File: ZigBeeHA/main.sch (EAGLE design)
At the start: 12 parts, among them IC1 REG1117

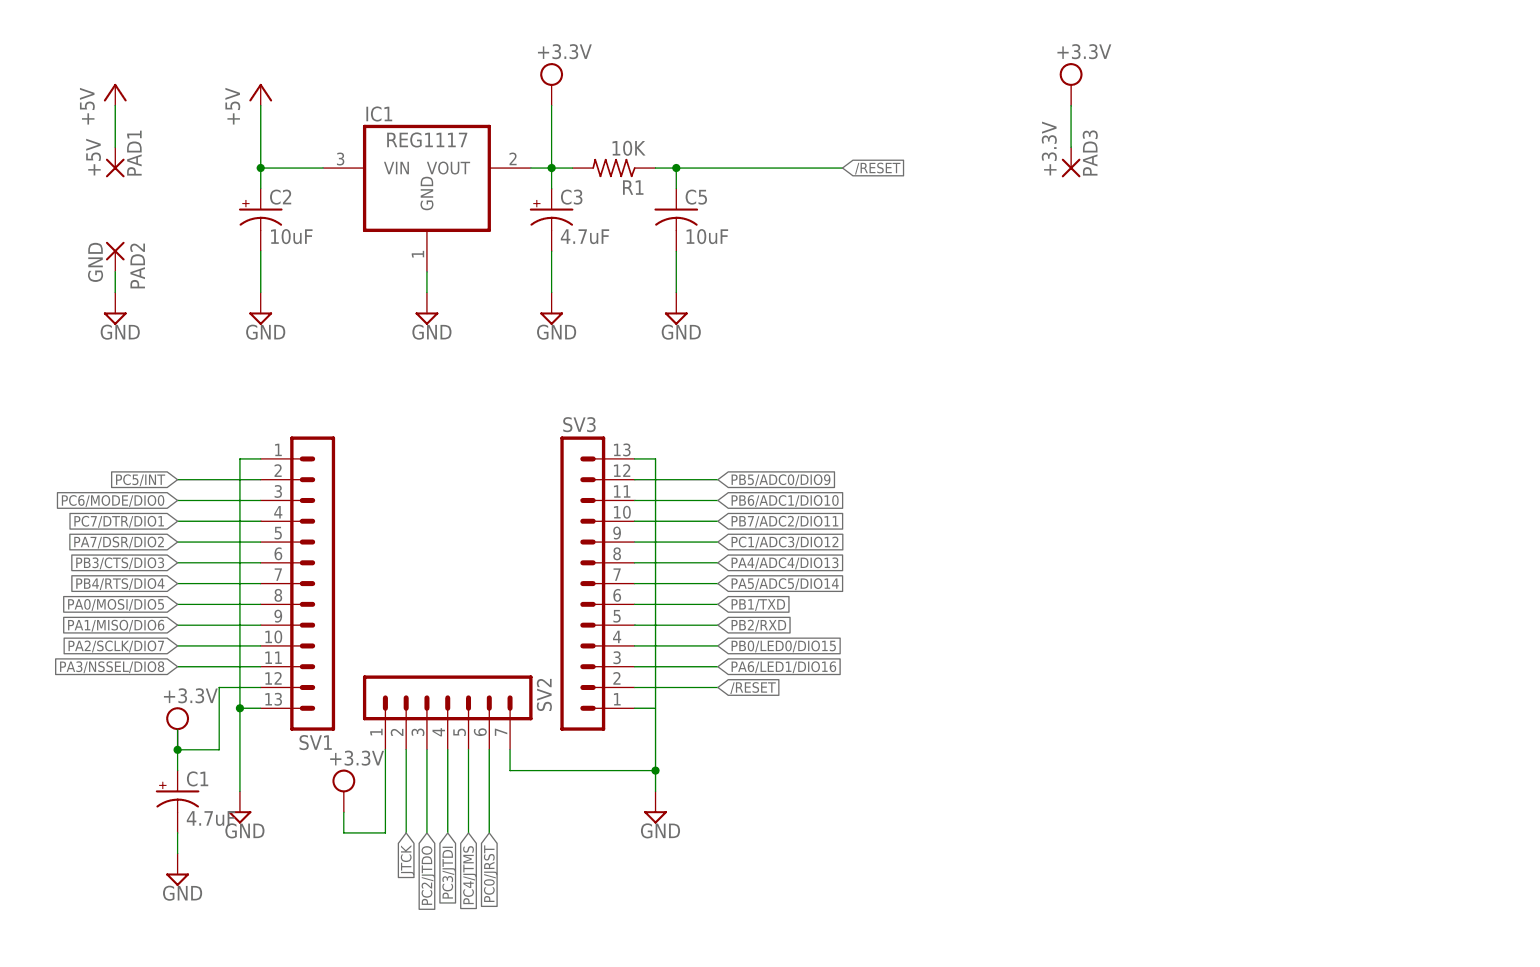
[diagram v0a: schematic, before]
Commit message: 1st completion
1st completion
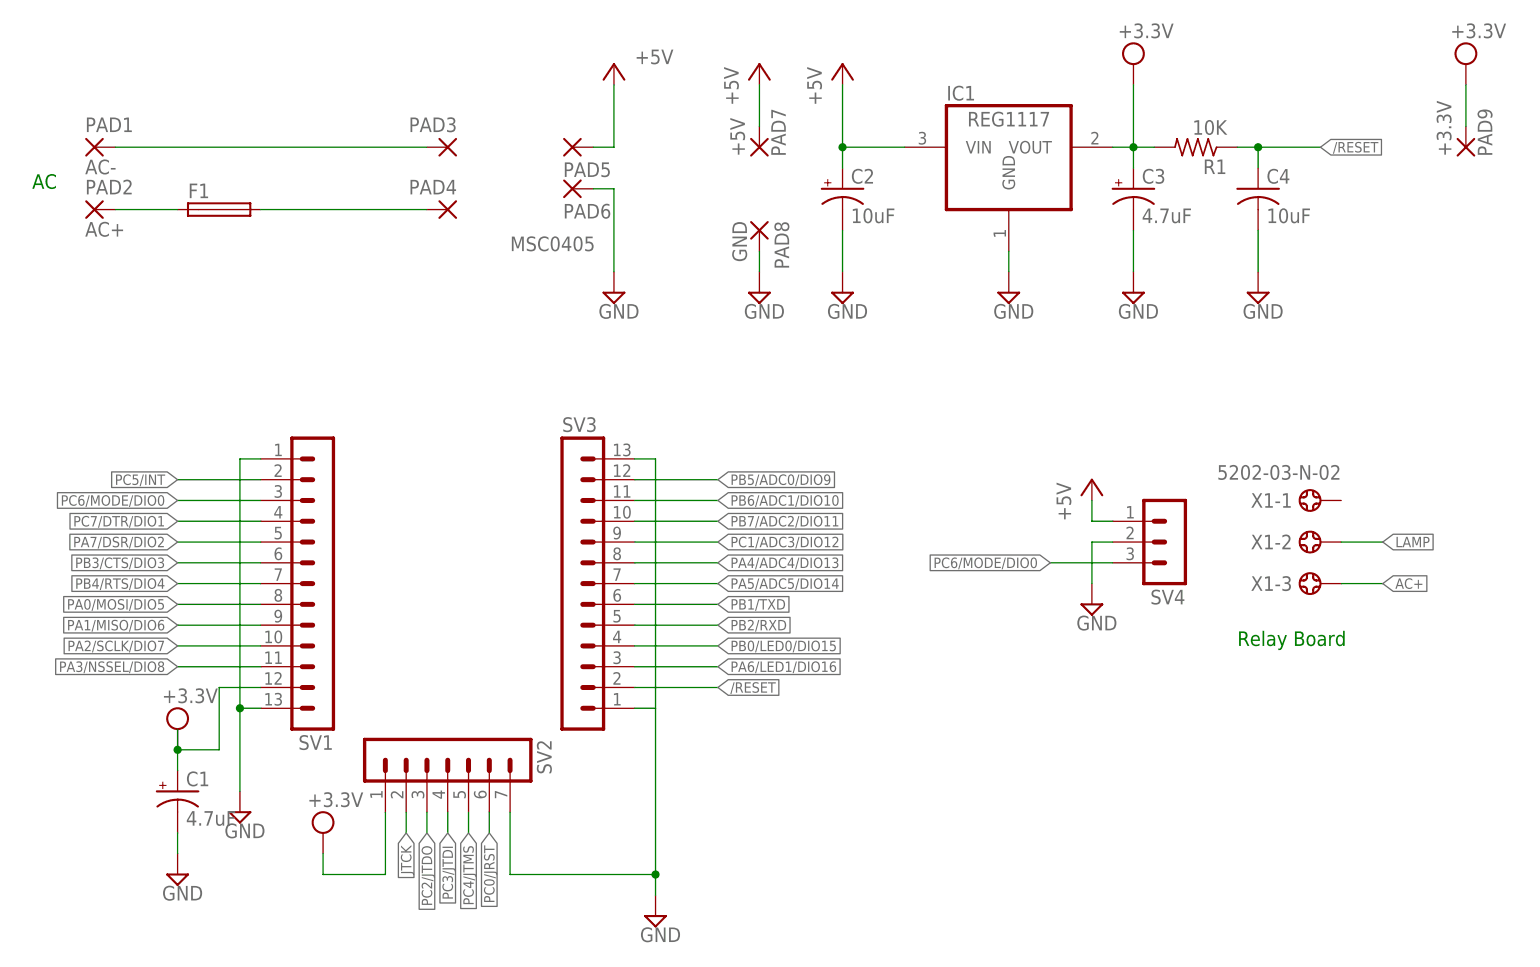
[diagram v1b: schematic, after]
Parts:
- removed C5: 10uF, rcl:C-USC1206
- added C4: 10uF, rcl:C-USC1206
- added F1: (no value), fuse:GSH15
- added PAD4, PAD5, PAD6: (no value), wirepad:2,54/0,8
- added PAD7: +5V, wirepad:2,54/0,8
- added PAD8: GND, wirepad:2,54/0,8
- added PAD9: +3.3V, wirepad:2,54/0,8
- added SV4: (no value), con-lstb:MA03-1
- added X1: 5202-03-N-02, con-ebyelectro:5202-03-N-02
- PAD1: value +5V -> AC-; device wirepad:2,54/0,8 -> wirepad:2,54/1,0
- PAD2: value GND -> AC+; device wirepad:2,54/0,8 -> wirepad:2,54/1,0
- PAD3: value +3.3V -> (none)
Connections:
- new net AC+: X1-3.1
- new net LAMP: X1-2.1
- new net N$1: PAD1.P, PAD3.P
- new net N$2: F1.1, PAD2.P
- new net N$3: F1.2, PAD4.P
- net +5V: now also PAD5.P, PAD7.P, SV4.1; no longer PAD1.P
- net /RESET: now also C4.1; no longer C5.1
- net GND: now also C4.2, PAD6.P, PAD8.P, SV4.2; no longer C5.2, PAD2.P
- net PC6/MODE/DIO0: now also SV4.3
- net VCC: now also PAD9.P; no longer PAD3.P
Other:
- note added: "AC"
- note added: "MSC0405"
- note added: "Relay Board"
- moved on the sheet: C2, C3, IC1, PAD1, PAD2, PAD3, R1, SV2
